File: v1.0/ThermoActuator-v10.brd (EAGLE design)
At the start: 101.6 x 53.3 mm, 28 parts, among them IC1 LM358D

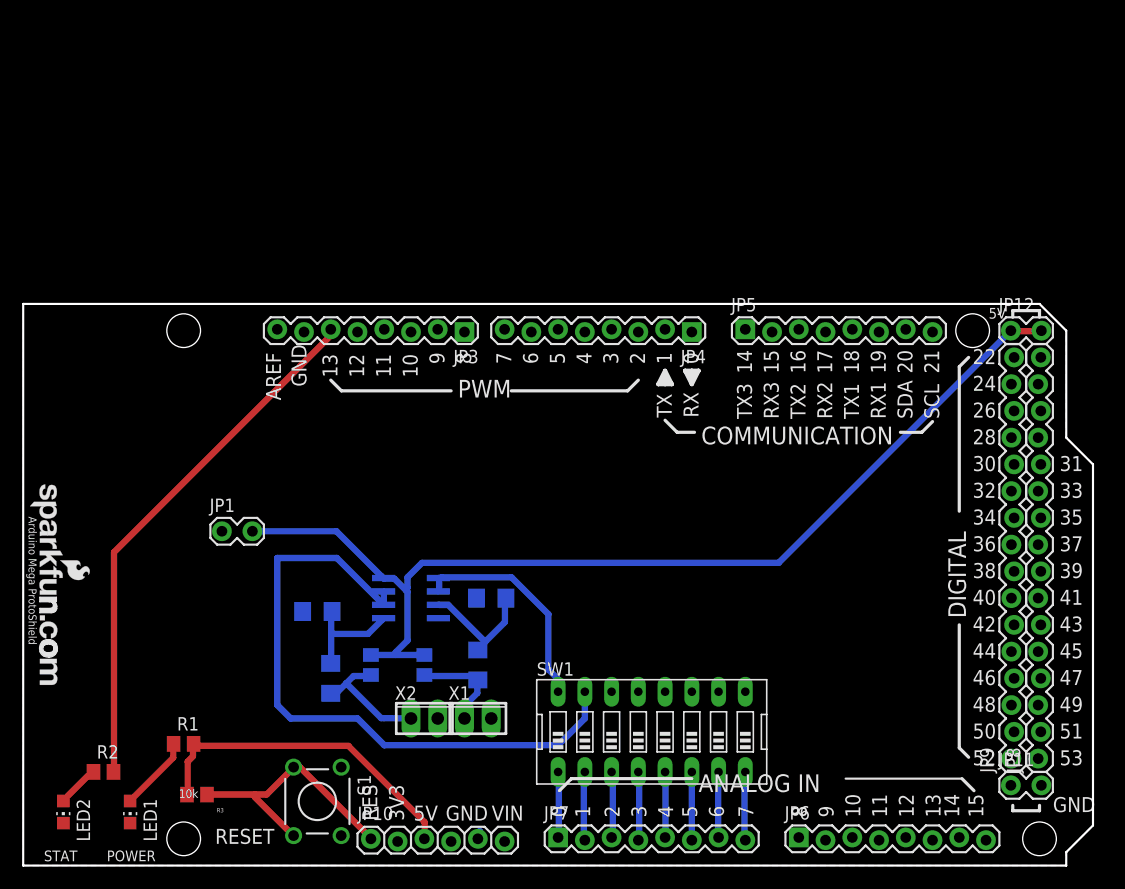
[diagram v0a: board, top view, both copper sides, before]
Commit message: shield centered
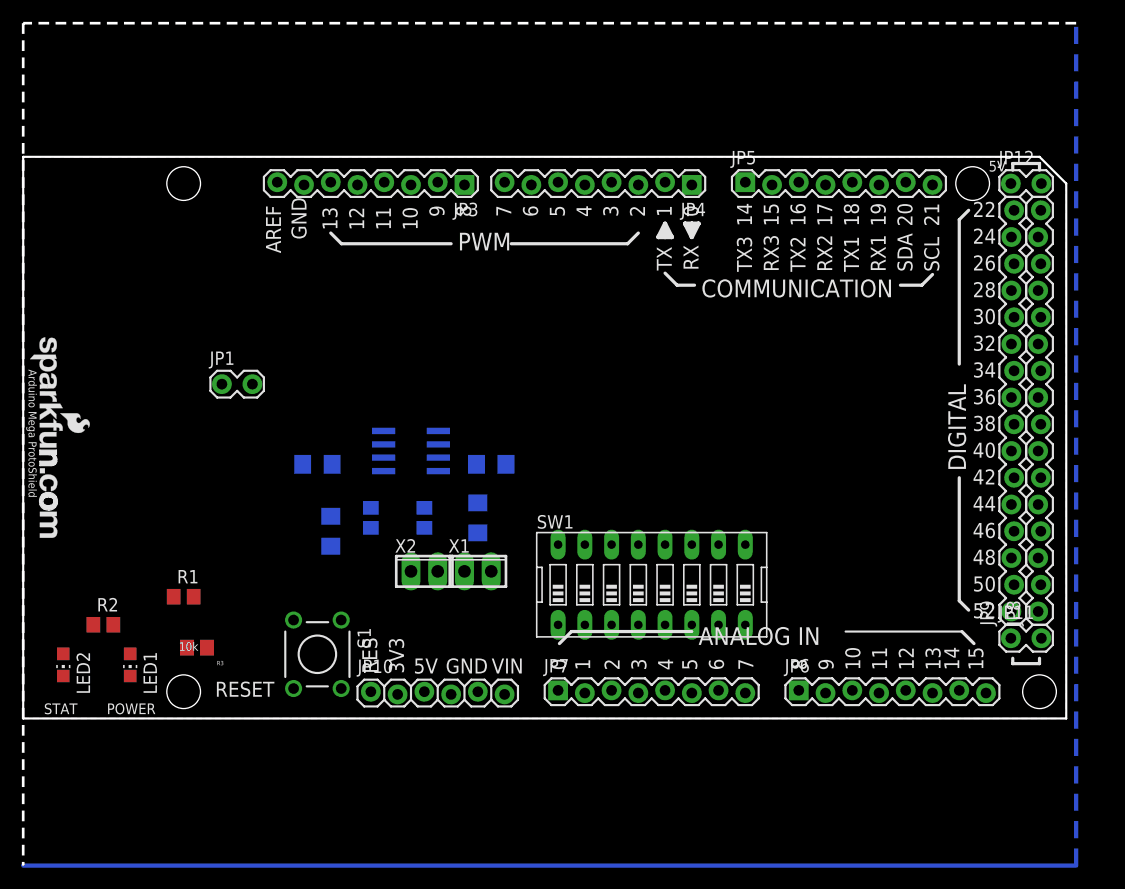
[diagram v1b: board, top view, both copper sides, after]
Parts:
- moved C2 14.0 mm to (27.9, 38.1)
- moved JP10 14.0 mm to (33.0, 16.5)
- moved JP6 14.0 mm to (73.7, 16.5)
- moved JP7 14.0 mm to (50.8, 16.5)
- moved R4 14.0 mm to (38.1, 33.0)
- moved R5 14.0 mm to (43.2, 33.0)
- moved R6 14.0 mm to (33.0, 33.0)
- moved SW1 14.0 mm to (59.7, 26.7)
- moved LED1 14.0 mm to (10.2, 19.1)
- moved LED2 14.0 mm to (3.81, 19.1)
- moved R1 14.0 mm to (15.2, 25.5)
- moved R3 14.0 mm to (16.5, 20.7)
- moved X1 14.0 mm to (43.2, 27.9)
- moved X2 14.0 mm to (38.1, 27.9)
- moved IC1 14.0 mm to (36.8, 39.4)
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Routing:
- net N$13: track 0.00 -> 180.0 mm
- net VDD: track 99.9 -> 0.00 mm
- net AS1: track 61.6 -> 0.00 mm
- net D13: track 50.6 -> 0.00 mm
- net 5V: track 31.7 -> 0.00 mm
- net RES: track 25.0 -> 0.00 mm
- net AS0: track 21.0 -> 0.00 mm
- net N$11: track 12.1 -> 0.00 mm
- net N$2: track 12.0 -> 0.00 mm
- net N$12: track 10.6 -> 0.00 mm
- net N$1: track 9.54 -> 0.00 mm
- net N$126: track 7.13 -> 0.00 mm
- net N$4: track 6.59 -> 0.00 mm
- net N$6: track 6.57 -> 0.00 mm
- net N$10: track 6.57 -> 0.00 mm
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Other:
- board size 101.6 x 53.3 mm -> 100 x 80 mm
- board text removed: "31"
- board text removed: "33"
- board text removed: "35"
- board text removed: "37"
- board text removed: "39"
- board text removed: "41"
- board text removed: "43"
- board text removed: "45"
- board text removed: "47"
- board text removed: "49"
- board text removed: "51"
- board text removed: "53"
